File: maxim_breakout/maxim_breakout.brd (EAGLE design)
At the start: 32.7 x 29.2 mm, 14 parts, among them U3 78M6612

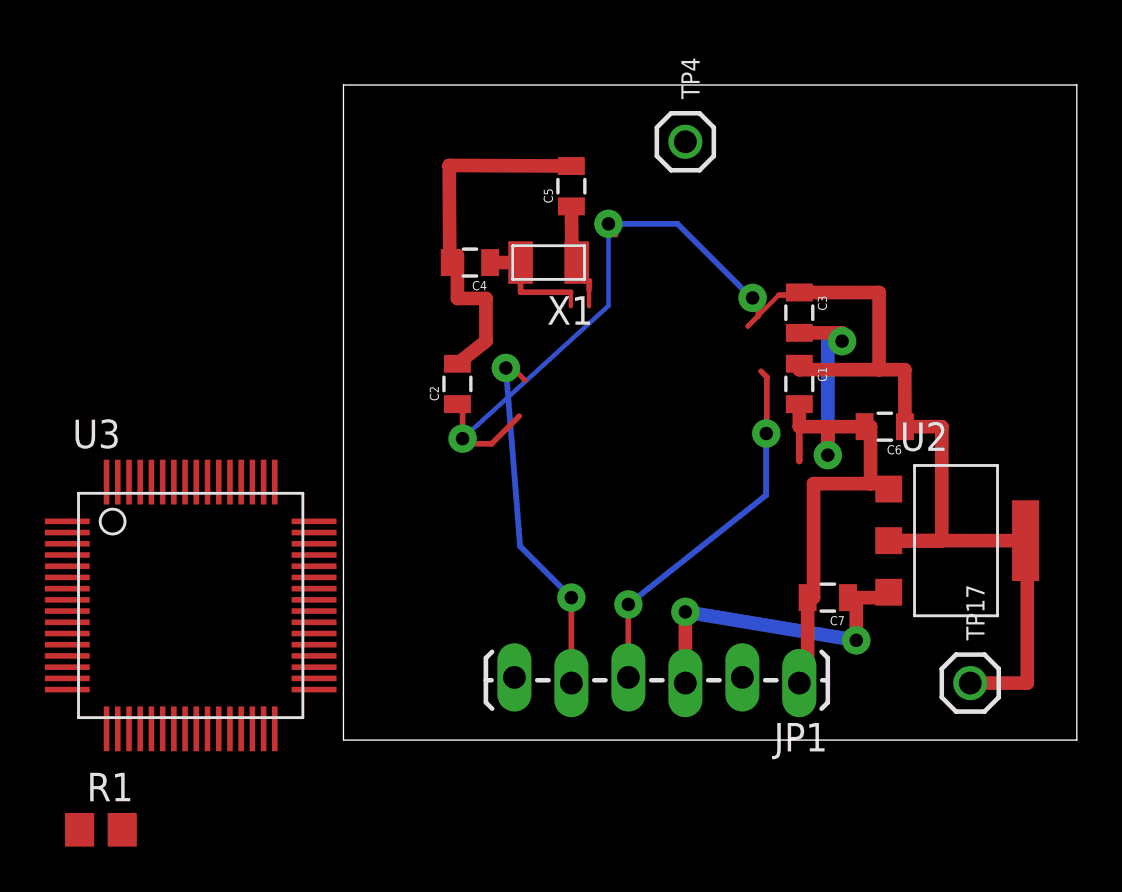
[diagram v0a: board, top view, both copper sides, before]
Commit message: Kevin's working on the board
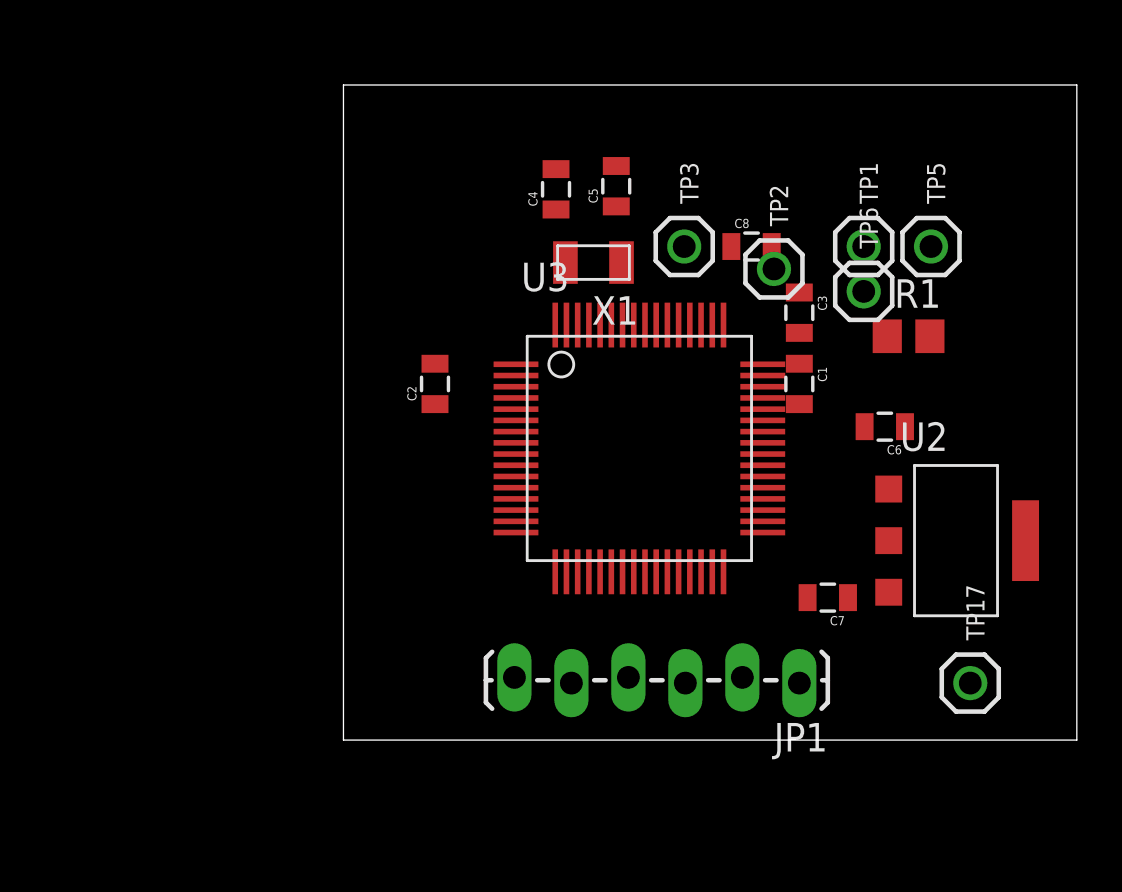
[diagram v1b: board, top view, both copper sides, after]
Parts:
- removed TP4: TESTPOINT100MIL, WSNlib:TESTPOINT-100MIL
- added C8: 33p, SparkFun:0805
- added TP1, TP2, TP3, TP5, TP6: TESTPOINT100MIL, WSNlib:TESTPOINT-100MIL
- moved R1 42.2 mm to (29.0, 18.0)
- moved U3 21.2 mm to (17.0, 13.0)
- moved C4 5.04 mm to (13.3, 24.6), turned to 90 degrees
- moved C5 2.00 mm to (16.0, 24.7)
- moved X1 2.00 mm to (15.0, 21.3)
- moved C2 1.00 mm to (7.89, 15.9)
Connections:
- new net N$4: C8.1, U3.47
- new net N$5: TP2.2, U3.54
- new net N$6: TP3.2, U3.53
- new net N$7: TP5.2, U3.51
- new net N$8: TP6.2, U3.52
- net GND: now also C8.2, TP1.2, U3.60
- net VCC: now also U3.50, U3.56, U3.9
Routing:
- net VCC: track 68.9 -> 0.00 mm, vias 3 -> 0
- net GND: track 47.9 -> 0.00 mm, vias 2 -> 0
- net RX_78: track 16.7 -> 0.00 mm, vias 2 -> 0
- net TX_78: track 16.1 -> 0.00 mm, vias 2 -> 0
- net N$1: track 15.2 -> 0.00 mm, vias 2 -> 0
- net N$12: track 5.54 -> 0.00 mm
- net N$13: track 4.76 -> 0.00 mm
